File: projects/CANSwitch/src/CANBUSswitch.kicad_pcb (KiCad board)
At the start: 2 copper layers, 19.9 x 6.1 mm, 5 parts, among them J1 Conn_01x02, J2 Conn_01x02

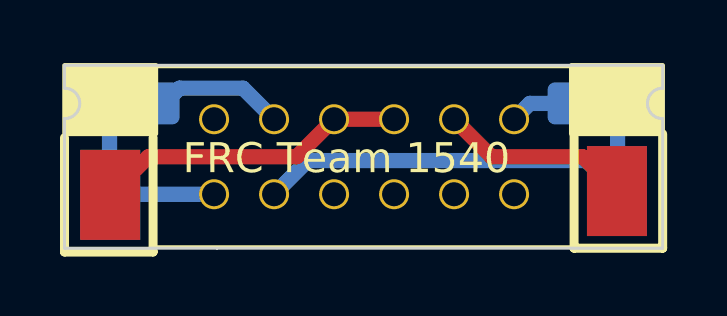
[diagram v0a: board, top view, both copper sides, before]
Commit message: Add files via upload
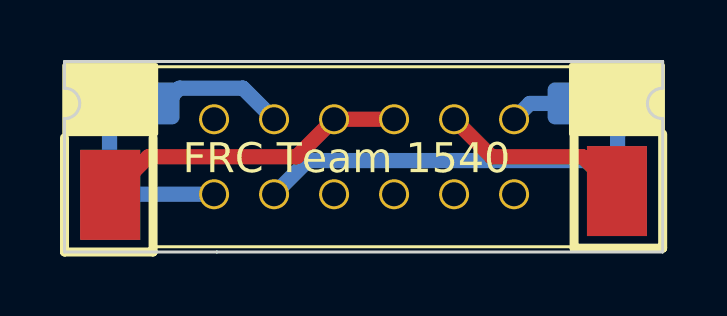
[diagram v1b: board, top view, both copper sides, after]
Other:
- board size 19.9 x 6.1 mm -> 19.9 x 6.4 mm
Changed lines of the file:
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@@
   (gr_line (start 201.549 38.862) (end 201.549 42.672)
     (stroke (width 0.3) (type solid)) (layer "F.SilkS"))
-  (gr_line (start 181.61 36.576) (end 201.549 36.576)
+  (gr_line (start 181.61 36.449) (end 201.549 36.449)
     (stroke (width 0.1) (type default)) (layer "Edge.Cuts"))
   (gr_arc (start 201.549 38.354) (mid 201.041 37.846) (end 201.549 37.338)
     (stroke (width 0.1) (type default)) (layer "Edge.Cuts"))
-  (gr_line (start 201.549 36.576) (end 201.549 37.338)
+  (gr_line (start 201.549 36.449) (end 201.549 37.338)
     (stroke (width 0.1) (type default)) (layer "Edge.Cuts"))
-  (gr_line (start 201.549 42.672) (end 186.69 42.672)
+  (gr_line (start 201.549 42.799) (end 186.69 42.799)
     (stroke (width 0.1) (type default)) (layer "Edge.Cuts"))
-  (gr_line (start 181.61 42.672) (end 181.61 38.354)
+  (gr_line (start 181.61 42.799) (end 181.61 38.354)
     (stroke (width 0.1) (type default)) (layer "Edge.Cuts"))
-  (gr_line (start 186.69 42.672) (end 181.61 42.672)
+  (gr_line (start 186.69 42.799) (end 181.61 42.799)
     (stroke (width 0.1) (type default)) (layer "Edge.Cuts"))
   (gr_arc (start 181.61 37.338) (mid 182.118 37.846) (end 181.61 38.354)
     (stroke (width 0.1) (type default)) (layer "Edge.Cuts"))
-  (gr_line (start 181.61 37.338) (end 181.61 36.576)
+  (gr_line (start 181.61 37.338) (end 181.61 36.449)
     (stroke (width 0.1) (type default)) (layer "Edge.Cuts"))
-  (gr_line (start 201.549 38.354) (end 201.549 42.672)
+  (gr_line (start 201.549 38.354) (end 201.549 42.799)
     (stroke (width 0.1) (type default)) (layer "Edge.Cuts"))
   (gr_text "Brendan Lee" (at 196.342 37.846) (layer "B.SilkS")
